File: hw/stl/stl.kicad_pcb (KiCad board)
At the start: 2 copper layers, 34 parts, among them J1 Screw_Terminal_01x04, Q1 IRF4905, Q2 IRFR5505TRLPBF, Q3 5505, Q4 5505, Q6 5505, Q7 5505, Q8 5505, U1 STM8S003F3P, U2 LM1117-3.3, U3 ULN2003A

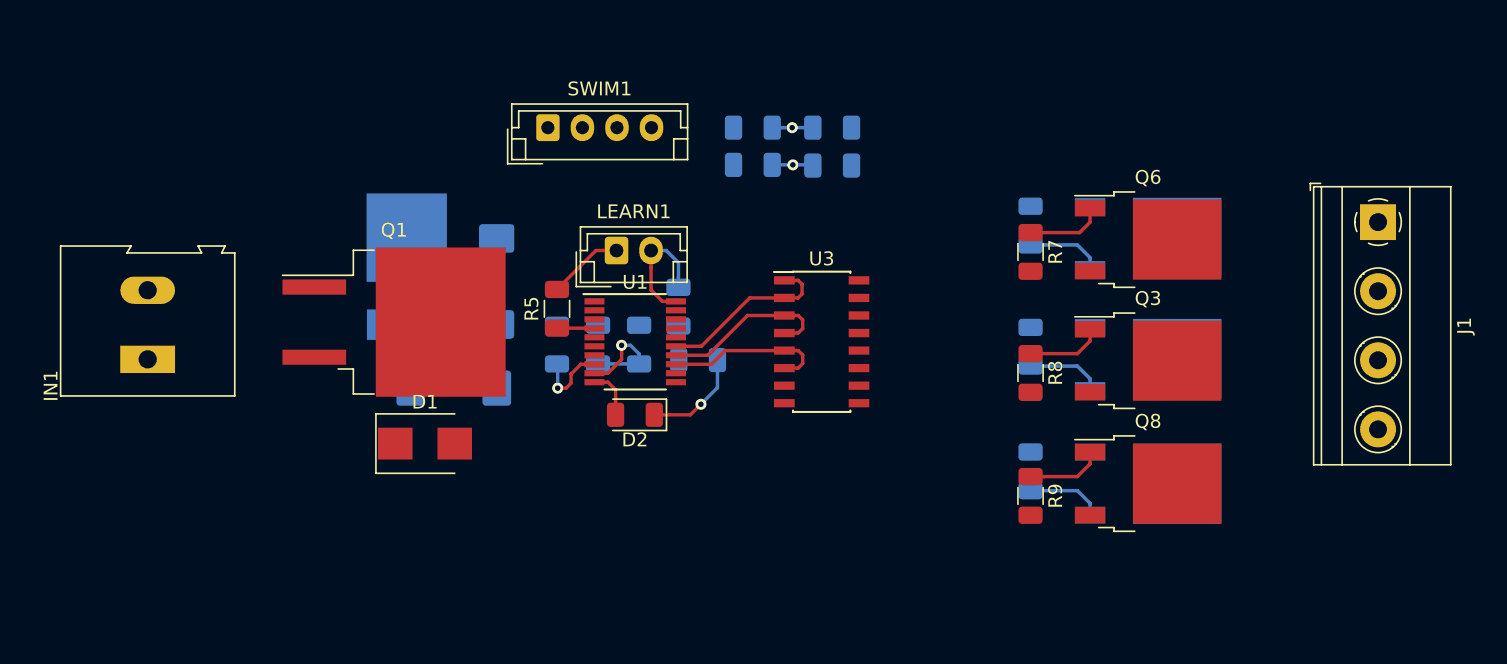
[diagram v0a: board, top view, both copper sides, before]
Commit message: WIP: draft tracing
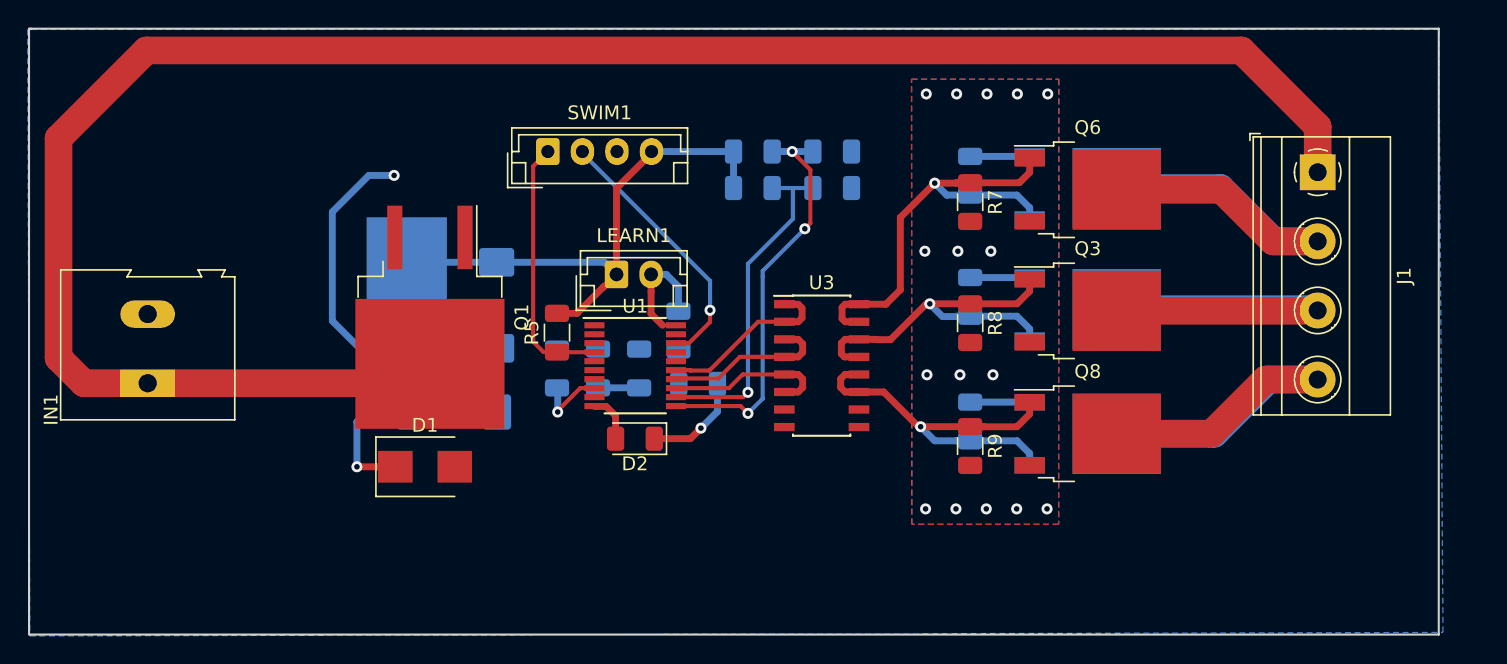
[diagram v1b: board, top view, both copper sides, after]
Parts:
- moved R2 5.98 mm to (231.1, 25.3), turned to 180 degrees
- moved R1 5.97 mm to (225.4, 25.3), turned to 180 degrees
- moved J1 5.67 mm to (266.3, 24.2)
- moved R11 5.67 mm to (241.1, 24.5)
- moved R12 5.67 mm to (241.1, 33.2)
- moved R13 5.67 mm to (241.1, 42.2)
- moved R7 5.67 mm to (241.1, 26.4)
- moved R8 5.67 mm to (241.1, 35.1)
- moved R9 5.67 mm to (241.1, 44.0)
- moved Q2 5.67 mm to (249.6, 25.3)
- moved Q3 5.67 mm to (249.6, 34.2)
- moved Q4 5.67 mm to (249.6, 43.1)
- moved Q6 5.67 mm to (249.6, 25.5)
- moved Q7 5.67 mm to (249.6, 34.1)
- moved Q8 5.67 mm to (249.6, 43.1)
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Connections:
- C4 pad 1: Net-(C4-Pad1) -> +12V
- D1 pad 1: Net-(C4-Pad1) -> +12V
- IN1 pad 1: +12V -> +BATT
- J1 pad 1: +12V -> +BATT
- Q1 pad 2: +12V -> +BATT
- Q1 pad 3: Net-(C4-Pad1) -> +12V
- U2 pad 3: Net-(C4-Pad1) -> +12V
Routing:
- net +BATT: track 0.00 -> 143.4 mm
- net +12V: track 0.00 -> 46.8 mm, vias 0 -> 18
- net lamp4_out: track 0.00 -> 32.3 mm
- net lamp2_out: track 0.00 -> 32.2 mm
- net lamp3_out: track 0.00 -> 29.1 mm
- net +3V3: track 14.1 -> 42.5 mm, vias 1 -> 0
- net CNT2: track 2.94 -> 29.7 mm, vias 1 -> 3
- net CNT1: track 2.96 -> 24.4 mm
- net lamp2_ctrl: track 11.2 -> 32.3 mm, vias 0 -> 1
- net SWIM: track 0.00 -> 19.3 mm, vias 0 -> 1
- net lamp4_ctrl: track 11.1 -> 27.7 mm, vias 0 -> 1
- net NRST: track 2.71 -> 18.9 mm
- net lamp3_ctrl: track 11.1 -> 27.0 mm, vias 0 -> 1
- added copper zone on B.Cu, net +12V
- added copper zone on F.Cu, net +12V
- added copper zone on B.Cu, net GND
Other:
- board outline added: 102 x 43.8 mm
- net class 12V added: clearance 0.2, trace_width 0.5, via_dia 0.8, via_drill 0.4
- net class 3v3 added: clearance 0.2, trace_width 0.5, via_dia 0.8, via_drill 0.4
- net class lamp added: clearance 0.2, trace_width 2, via_dia 0.8, via_drill 0.4
- net class signalling removed
- net class signals added: clearance 0.2, trace_width 0.3, via_dia 0.8, via_drill 0.4
